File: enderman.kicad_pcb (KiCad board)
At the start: 2 copper layers, 29 x 98 mm, 21 parts, among them SW1 SW_SPDT, U1 LM556

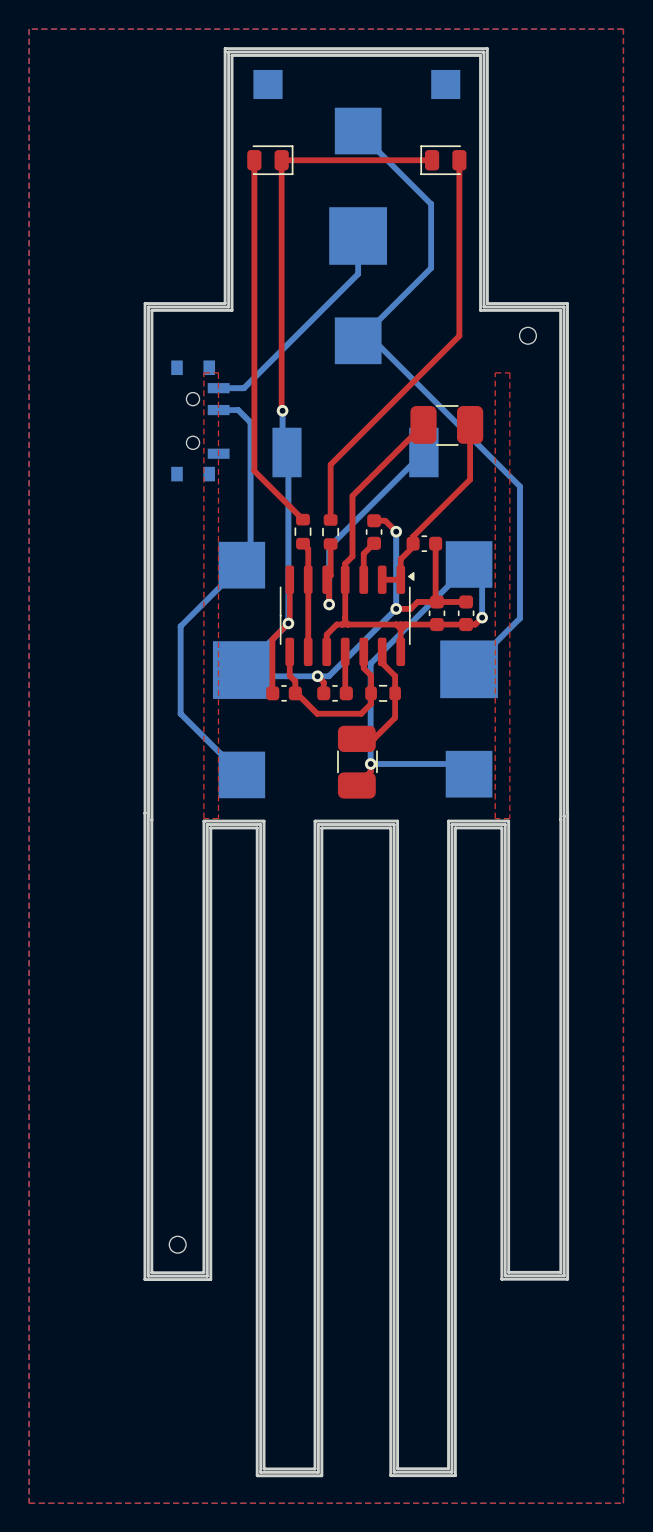
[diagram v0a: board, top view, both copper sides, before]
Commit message: atari punk version
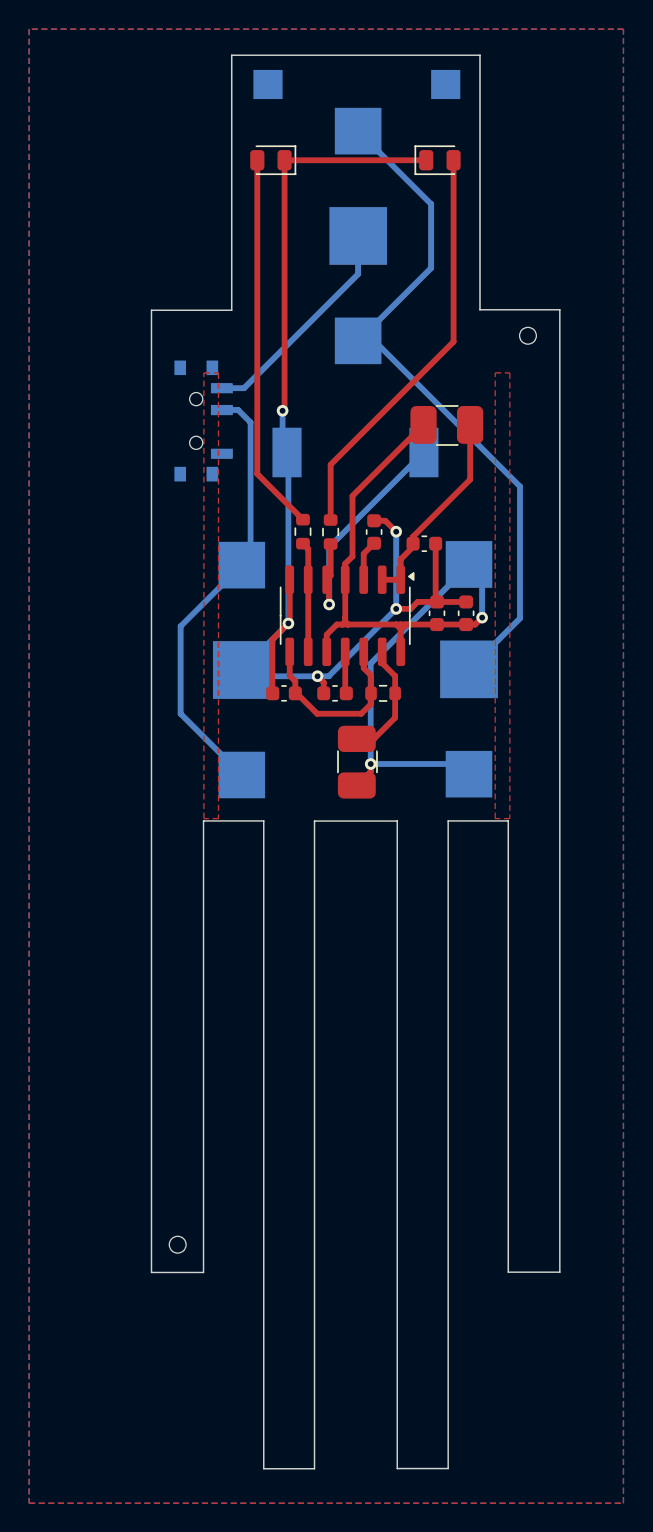
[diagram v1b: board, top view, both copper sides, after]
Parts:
- moved D2 0.40 mm to (144.4, 47.2)
- moved SW1 0.22 mm to (128.0, 65.1)
- moved D1 0.20 mm to (132.8, 47.2)
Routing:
- net GND: track 85.4 -> 84.8 mm
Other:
- board size 29 x 98 mm -> 28 x 97 mm
